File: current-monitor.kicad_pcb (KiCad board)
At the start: 4 copper layers, 70 x 58.2 mm, 152 parts, among them J201 CONN-3, J601 USB-MICROB, J602 SWD, J603 CONN-6, K201 RELAY-DPDT-EE2-SPLIT, K202 RELAY-DPDT-EE2-SPLIT, Q201 DRDC3105E6, U201 FSA1259A, U202 MAX4737EUD, U301 AD8429A, U302 TL032C, U303 LM833, U401 INA826, U501 TL032C, U601 K22F-64LQFP, U701 LM27313, U702 MAX6070, U703 LTC3260MSE, Y601 4MHz

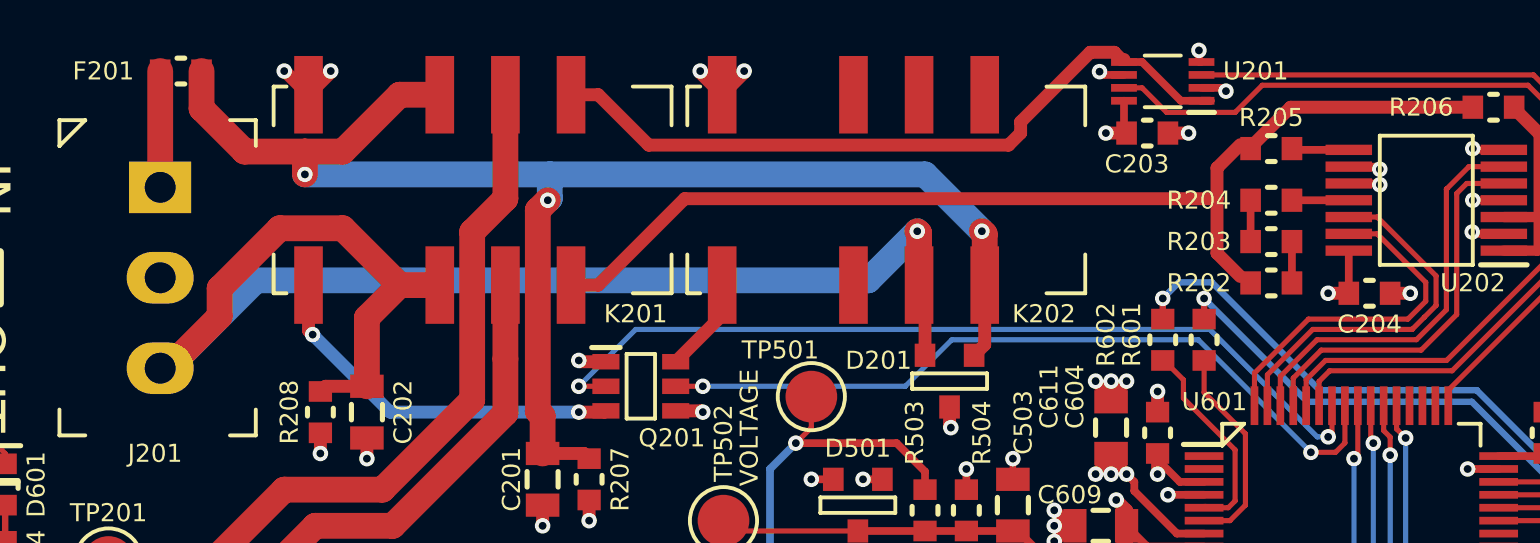
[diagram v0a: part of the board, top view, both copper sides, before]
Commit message: zone connections
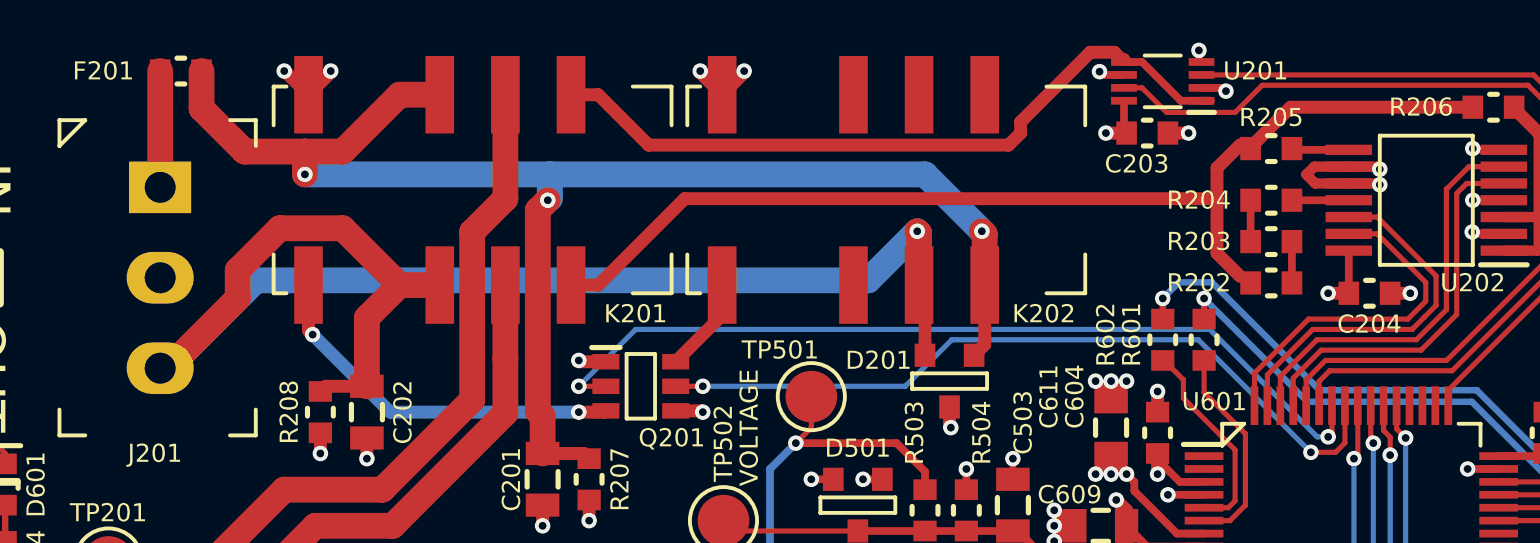
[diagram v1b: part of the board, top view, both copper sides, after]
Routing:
- net COM: track 111.3 -> 114.9 mm
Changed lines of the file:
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@@
     (thickness 1.6)
     (drawings 14)
-    (tracks 1240)
+    (tracks 1244)
     (zones 0)
     (modules 152)
@@
       (net 12 +3.00V))
     (pad 15 smd rect (at -5.7 3.25) (size 1.5 0.3) (layers F.Cu F.Paste F.Mask)
-      (net 2 COM))
+      (net 2 COM) (zone_connect 1))
     (pad 16 smd rect (at -5.7 3.75) (size 1.5 0.3) (layers F.Cu F.Paste F.Mask)
-      (net 2 COM))
+      (net 2 COM) (zone_connect 1))
     (pad 17 smd rect (at -3.75 5.7 90) (size 1.5 0.3) (layers F.Cu F.Paste F.Mask))
     (pad 18 smd rect (at -3.25 5.7 90) (size 1.5 0.3) (layers F.Cu F.Paste F.Mask)
@@
       (net 78 "Net-(R205-Pad2)"))
     (pad 9 smd rect (at 1.3 -3 90) (size 0.4 1.8) (layers F.Cu F.Paste F.Mask)
-      (net 2 COM))
+      (net 2 COM) (zone_connect 1))
     (pad 10 smd rect (at 0.65 -3 90) (size 0.4 1.8) (layers F.Cu F.Paste F.Mask)
-      (net 2 COM))
+      (net 2 COM) (zone_connect 1))
     (pad 11 smd rect (at 0 -3 90) (size 0.4 1.8) (layers F.Cu F.Paste F.Mask)
       (net 77 "Net-(R204-Pad2)"))
@@
   (segment (start 102.75 87.8) (end 102.5 87.55) (width 0.4) (layer F.Cu) (net 1) (status 30))
   (segment (start 102.5 85.25) (end 103.05 84.7) (width 0.4) (layer F.Cu) (net 1) (status 30))
+  (segment (start 145.8 66.7) (end 144.468202 66.7) (width 0.4) (layer F.Cu) (net 2))
+  (segment (start 144.468202 66.7) (end 144.168202 67) (width 0.4) (layer F.Cu) (net 2))
+  (segment (start 145.8 67.35) (end 144.5 67.35) (width 0.4) (layer F.Cu) (net 2))
+  (segment (start 144.5 67.35) (end 144.15 67) (width 0.4) (layer F.Cu) (net 2))
+  (segment (start 145.8 67.35) (end 146.95 67.35) (width 0.4) (layer F.Cu) (net 2))
+  (segment (start 146.95 67.35) (end 147 67.4) (width 0.4) (layer F.Cu) (net 2))
+  (segment (start 145.8 66.7) (end 146.9 66.7) (width 0.4) (layer F.Cu) (net 2))
+  (segment (start 146.9 66.7) (end 147 66.8) (width 0.4) (layer F.Cu) (net 2))
   (segment (start 140.3 97.5) (end 140.3 98.3) (width 0.2) (layer F.Cu) (net 2))
   (segment (start 140.3 98.3) (end 140.2 98.4) (width 0.2) (layer F.Cu) (net 2))
@@
   (segment (start 138.8 65.4) (end 139.6 65.4) (width 0.5) (layer F.Cu) (net 2) (status 10))
   (via (at 139.6 65.4) (size 0.6) (drill 0.3) (layers F.Cu B.Cu) (net 2))
-  (segment (start 145.8 66.7) (end 146.9 66.7) (width 0.3) (layer F.Cu) (net 2) (status 10))
-  (segment (start 146.9 66.7) (end 147 66.8) (width 0.3) (layer F.Cu) (net 2))
   (via (at 147 66.8) (size 0.6) (drill 0.3) (layers F.Cu B.Cu) (net 2))
-  (segment (start 145.8 67.35) (end 146.95 67.35) (width 0.3) (layer F.Cu) (net 2) (status 10))
-  (segment (start 146.95 67.35) (end 147 67.4) (width 0.3) (layer F.Cu) (net 2))
   (via (at 147 67.4) (size 0.6) (drill 0.3) (layers F.Cu B.Cu) (net 2))
   (segment (start 151.8 66.05) (end 150.65 66.05) (width 0.3) (layer F.Cu) (net 2) (status 10))
@@
   (segment (start 131.7 71.273) (end 131.71 71.283) (width 1) (layer F.Cu) (net 73) (status 30))
   (segment (start 131.71 70.338) (end 131.71 71.283) (width 1) (layer F.Cu) (net 73) (status 30))
+  (segment (start 99.8 74.5) (end 100.1 74.5) (width 1) (layer F.Cu) (net 74))
+  (segment (start 100.1 74.5) (end 102.8 71.8) (width 1) (layer F.Cu) (net 74))
+  (segment (start 106.865999 69.083999) (end 109.065 71.283) (width 1) (layer F.Cu) (net 74))
+  (segment (start 102.8 71.8) (end 102.8 70.709798) (width 1) (layer F.Cu) (net 74))
+  (segment (start 102.8 70.709798) (end 104.425799 69.083999) (width 1) (layer F.Cu) (net 74))
+  (segment (start 104.425799 69.083999) (end 106.865999 69.083999) (width 1) (layer F.Cu) (net 74))
   (segment (start 106.2 75.2) (end 106 75.4) (width 0.5) (layer F.Cu) (net 74))
   (segment (start 107.8 75.2) (end 106.2 75.2) (width 0.5) (layer F.Cu) (net 74))
@@
   (segment (start 103.5 71.1) (end 100.1 74.5) (width 1) (layer B.Cu) (net 74))
   (segment (start 100.1 74.5) (end 99.8 74.5) (width 1) (layer B.Cu) (net 74))
-  (segment (start 99.8 74.5) (end 100.1 74.5) (width 1) (layer F.Cu) (net 74))
-  (segment (start 100.1 74.5) (end 102.1 72.5) (width 1) (layer F.Cu) (net 74))
-  (segment (start 102.1 72.5) (end 102.1 71.409798) (width 1) (layer F.Cu) (net 74))
-  (segment (start 104.425799 69.083999) (end 106.865999 69.083999) (width 1) (layer F.Cu) (net 74))
-  (segment (start 102.1 71.409798) (end 104.425799 69.083999) (width 1) (layer F.Cu) (net 74))
   (segment (start 129.4 74) (end 129.4 71.513) (width 0.5) (layer F.Cu) (net 74))
   (segment (start 129.4 71.513) (end 129.17 71.283) (width 0.5) (layer F.Cu) (net 74))
   (segment (start 129.1 69.2) (end 127.2 71.1) (width 1) (layer B.Cu) (net 74))
-  (segment (start 106.865999 69.083999) (end 109.065 71.283) (width 1) (layer F.Cu) (net 74))
   (segment (start 109.065 71.283) (end 110.62 71.283) (width 1) (layer F.Cu) (net 74) (status 20))
   (segment (start 129.17 71.283) (end 129.17 69.27) (width 1) (layer F.Cu) (net 74) (status 10))
@@
     (connect_pads yes (clearance 0.2))
     (min_thickness 0.254)
-    (fill yes (arc_segments 32) (thermal_gap 0.508) (thermal_bridge_width 0.508))
+    (fill yes (arc_segments 32) (thermal_gap 0.2) (thermal_bridge_width 0.508))
     (polygon
       (pts
